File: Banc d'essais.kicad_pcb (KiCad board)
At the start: 2 copper layers, 3 parts, among them U1 MCP4431-xxxx-ST

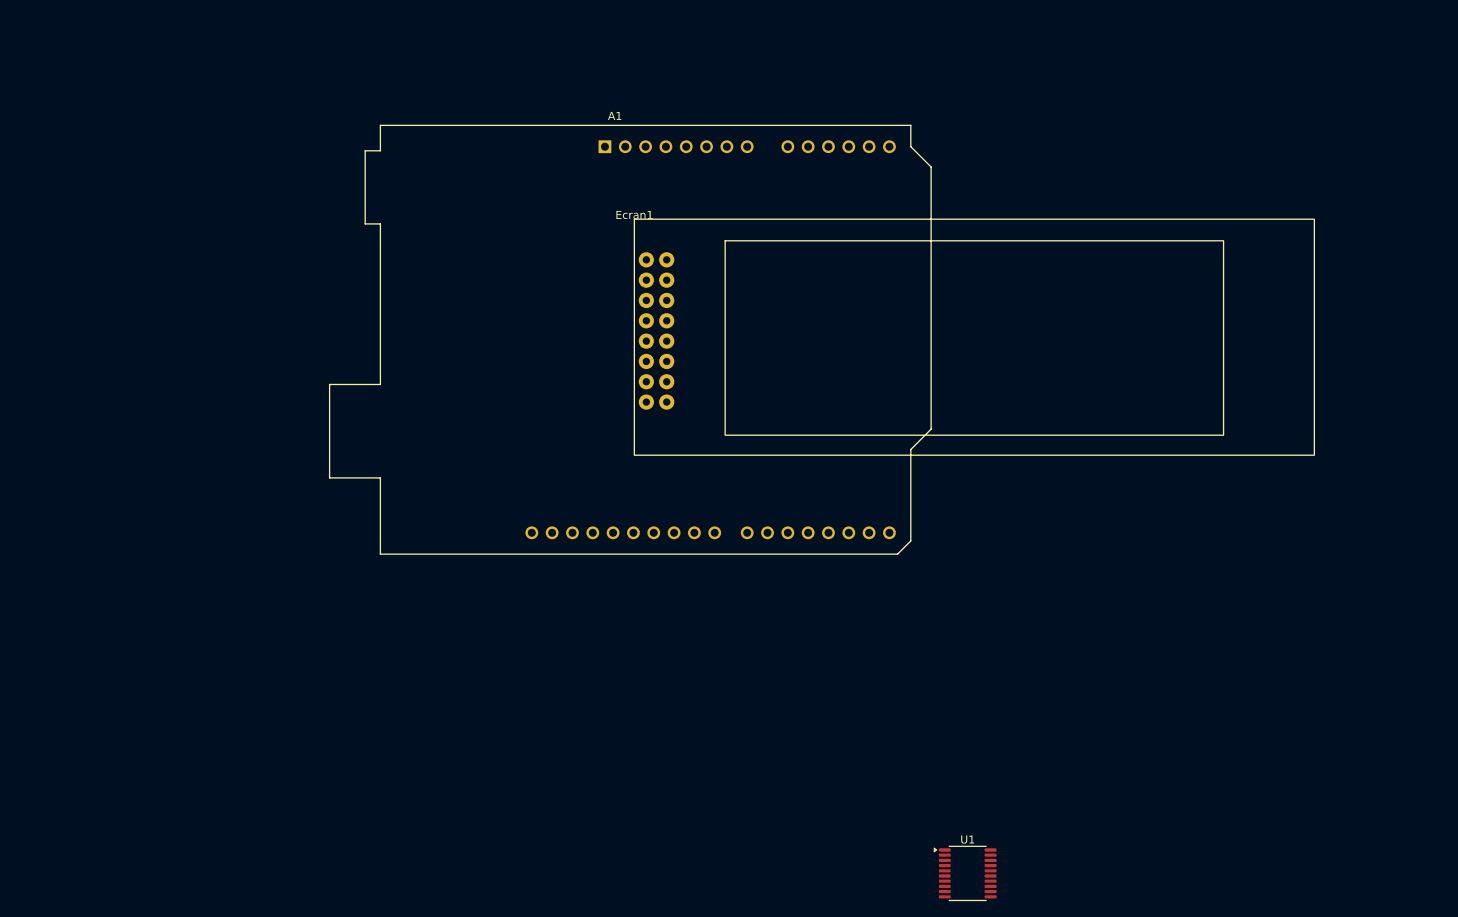
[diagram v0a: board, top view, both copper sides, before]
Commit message: modification + finalisation du PCB et du schéma
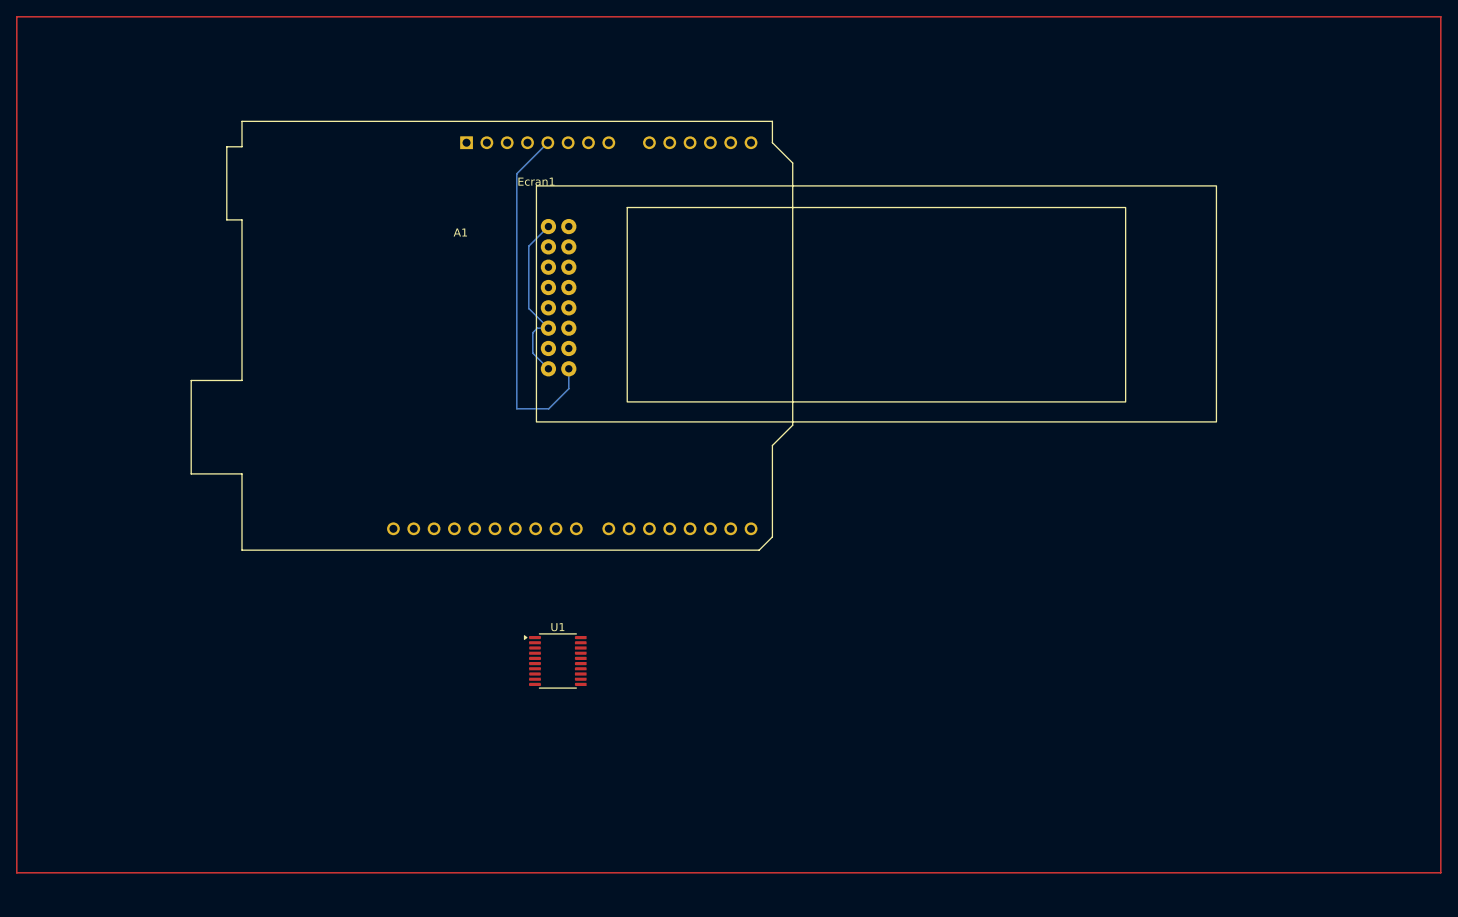
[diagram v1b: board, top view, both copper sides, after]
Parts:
- moved U1 57.7 mm to (142.1, 114.5)
- moved A1 17.3 mm to (130.7, 49.7)
- moved Ecran1 12.9 mm to (139.5, 55.1)
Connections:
- net Earth renamed Net-(Ecran1-K)
- A1 pad 11: Net-(A1-A2) -> unconnected-(A1-A2-Pad11)
- A1 pad 12: Net-(A1-A3) -> unconnected-(A1-A3-Pad12)
- A1 pad 2: Net-(A1-IOREF) -> unconnected-(A1-IOREF-Pad2)
- A1 pad 3: Net-(A1-+5V) -> unconnected-(A1-~{RESET}-Pad3)
- A1 pad 4: Net-(A1-+5V) -> unconnected-(A1-3V3-Pad4)
- Ecran1 pad 12: Net-(A1-+5V) -> unconnected-(Ecran1-DB5-Pad12)
- Ecran1 pad 13: Net-(A1-+5V) -> unconnected-(Ecran1-DB6-Pad13)
- Ecran1 pad 14: Net-(A1-IOREF) -> unconnected-(Ecran1-DB7-Pad14)
- Ecran1 pad 4: Net-(A1-A3) -> unconnected-(Ecran1-RS-Pad4)
- Ecran1 pad 6: Net-(A1-A2) -> unconnected-(Ecran1-E-Pad6)
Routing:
- net Net-(A1-+5V): track 0.00 -> 44.9 mm
- net Net-(Ecran1-K): track 0.00 -> 22.2 mm
